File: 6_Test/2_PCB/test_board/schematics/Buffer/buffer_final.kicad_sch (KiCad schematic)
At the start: 15 parts, among them U1 SN74ALVCH162827DLR

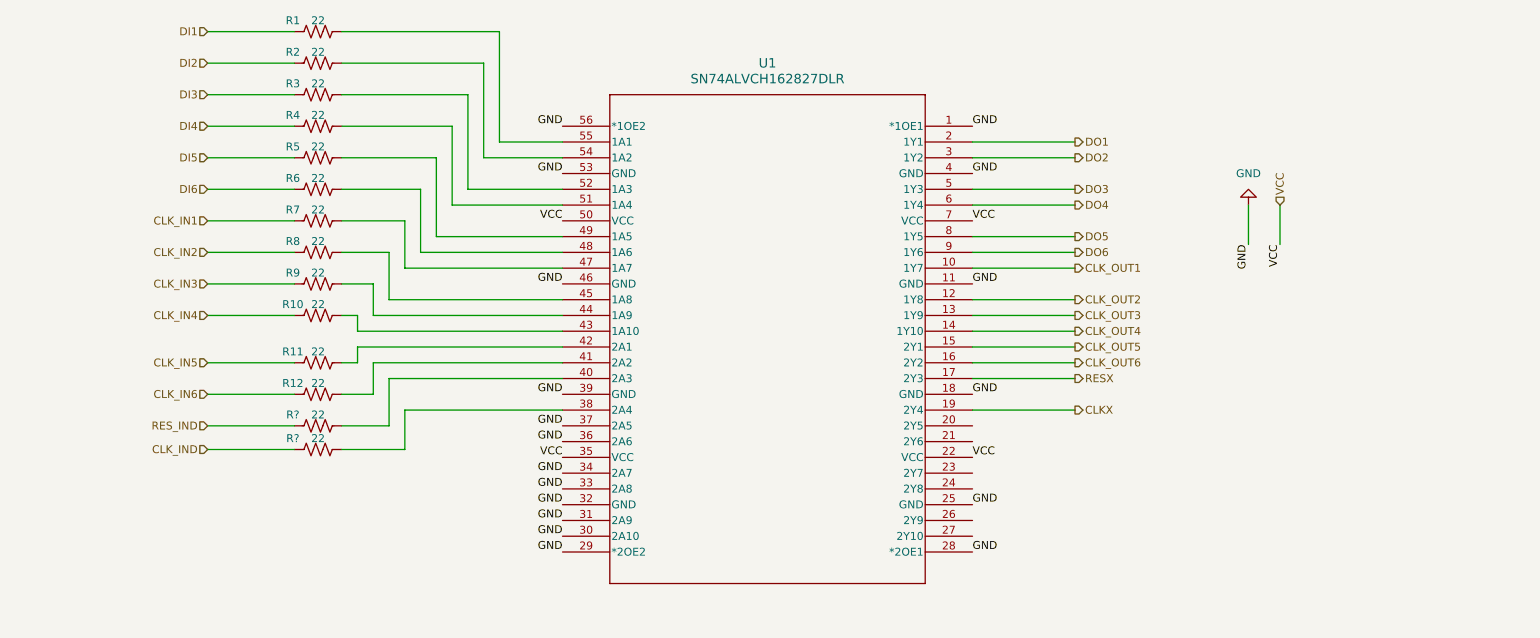
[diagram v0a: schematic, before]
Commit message: Edits 112524
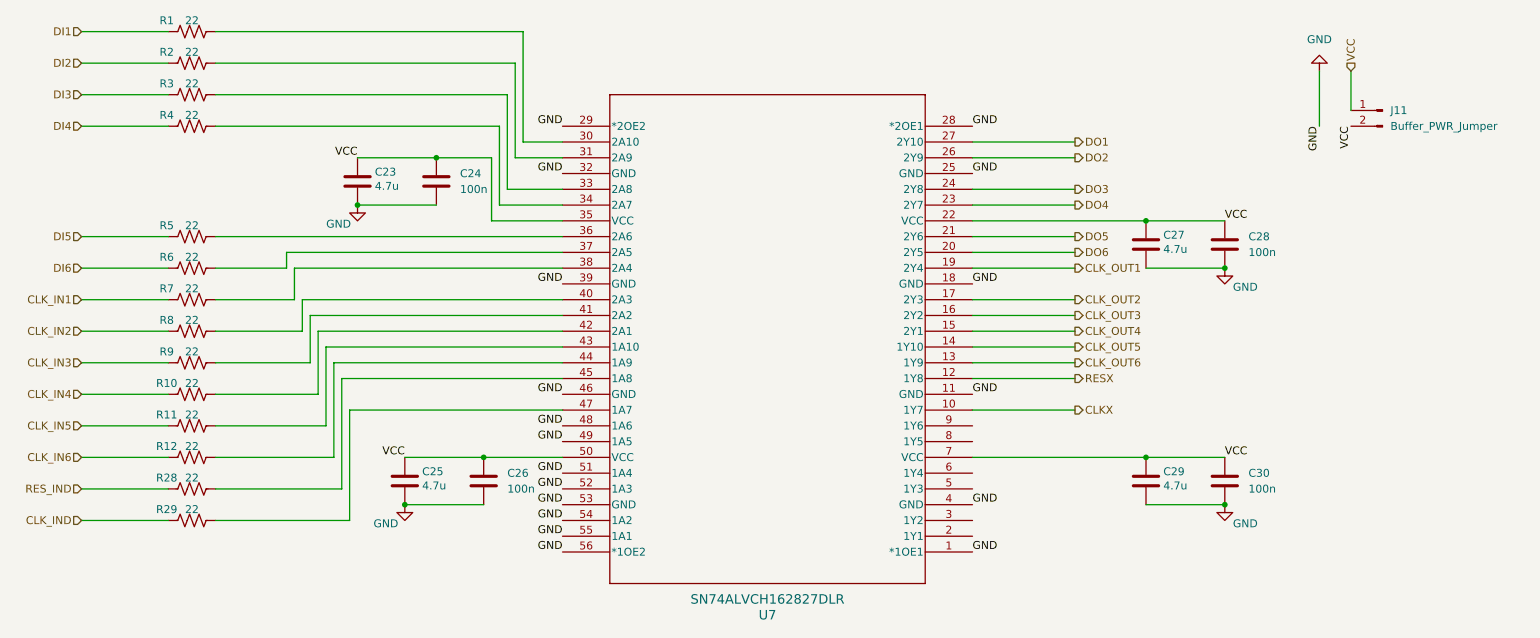
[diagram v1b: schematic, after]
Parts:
- removed U1: SN74ALVCH162827DLR, DL56, symbol 74ALVCH:SN74ALVCH162827DLR
- added C23, C25, C27, C29: 4.7u, Cap4.7uFFootprints:CAP_0603_CL10A_1P6XP8_SAM, symbol Device:C
- added C24, C26, C28, C30: 100n, cap100nFFootprints:CAP_CL05_SAM, symbol Device:C
- added J11: Buffer_PWR_Jumper, Connector_PinHeader_2.54mm:PinHeader_1x02_P2.54mm_Vertical, symbol Connector:Conn_01x02_Pin
- added U7: SN74ALVCH162827DLR, 74ALVCHFootprints:DL56, symbol 74ALVCH:SN74ALVCH162827DLR
- gave numbers to parts that had none: 2
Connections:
- net CLKX: now also U7.10 (1Y7)
- net CLK_OUT1: now also U7.19 (2Y4)
- net CLK_OUT2: now also U7.17 (2Y3)
- net CLK_OUT3: now also U7.16 (2Y2)
- net CLK_OUT4: now also U7.15 (2Y1)
- net CLK_OUT5: now also U7.14 (1Y10)
- net CLK_OUT6: now also U7.13 (1Y9)
- net DO1: now also U7.27 (2Y10)
- net DO2: now also U7.26 (2Y9)
- net DO3: now also U7.24 (2Y8)
- net DO4: now also U7.23 (2Y7)
- net DO5: now also U7.21 (2Y6)
- net DO6: now also U7.20 (2Y5)
- net GND: now also C23.2, C24.2, C25.2, C26.2, C27.2, C28.2, C29.2, C30.2, U7.1 (*1OE1), U7.11 (GND), U7.18 (GND), U7.25 (GND), U7.28 (*2OE1), U7.29 (*2OE2), U7.32 (GND), U7.39 (GND), U7.4 (GND), U7.46 (GND), U7.48 (1A6), U7.49 (1A5), U7.51 (1A4), U7.52 (1A3), U7.53 (GND), U7.54 (1A2), U7.55 (1A1), U7.56 (*1OE2)
- net RESX: now also U7.12 (1Y8)
- net VCC: now also C23.1, C24.1, C25.1, C26.1, C27.1, C28.1, C29.1, C30.1, J11.1 (Pin_1), J11.2 (Pin_2), U7.22 (VCC), U7.35 (VCC), U7.50 (VCC), U7.7 (VCC)
- net at R2.2: now also U7.31 (2A9)
- net at R11.2: now also U7.43 (1A10)
- net at R1.2: now also U7.30 (2A10)
- net at R4.2: now also U7.34 (2A7)
- net at R6.2: now also U7.37 (2A5)
- net at R12.2: now also U7.44 (1A9)
- net at R5.2: now also U7.36 (2A6)
- net at R9.2: now also U7.41 (2A2)
- net at R10.2: now also U7.42 (2A1)
- net at R7.2: now also U7.38 (2A4)
- net at R3.2: now also U7.33 (2A8)
- net at R29.2: now also U7.47 (1A7)
- net at R28.2: now also U7.45 (1A8)
- net at R8.2: now also U7.40 (2A3)
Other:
- moved on the sheet: R1, R10, R11, R12, R2, R28, R29, R3, R4, R5, R6, R7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
